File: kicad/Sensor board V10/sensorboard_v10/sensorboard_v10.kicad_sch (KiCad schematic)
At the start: 61 parts, among them J1 Conn_01x02, J10 Conn_01x04, J11 Conn_01x02, J19 Conn_01x03, J2 USB_C_Receptacle_USB2.0_14P, J20 Conn_01x02, J21 Conn_01x06, J3 Conn_01x02, J6 Conn_01x04, J7 Conn_01x04, Q1 MMBT3904, Q2 MMBT3904, SW1 SW_SPST, SW2 SW_SPST, U1 ESP32-S3-WROOM-2, U2 CH340C, U3 TJA1051T-3, U4 LM2576S-5, U5 AMS1117-3.3, U7 TXS0102DCU

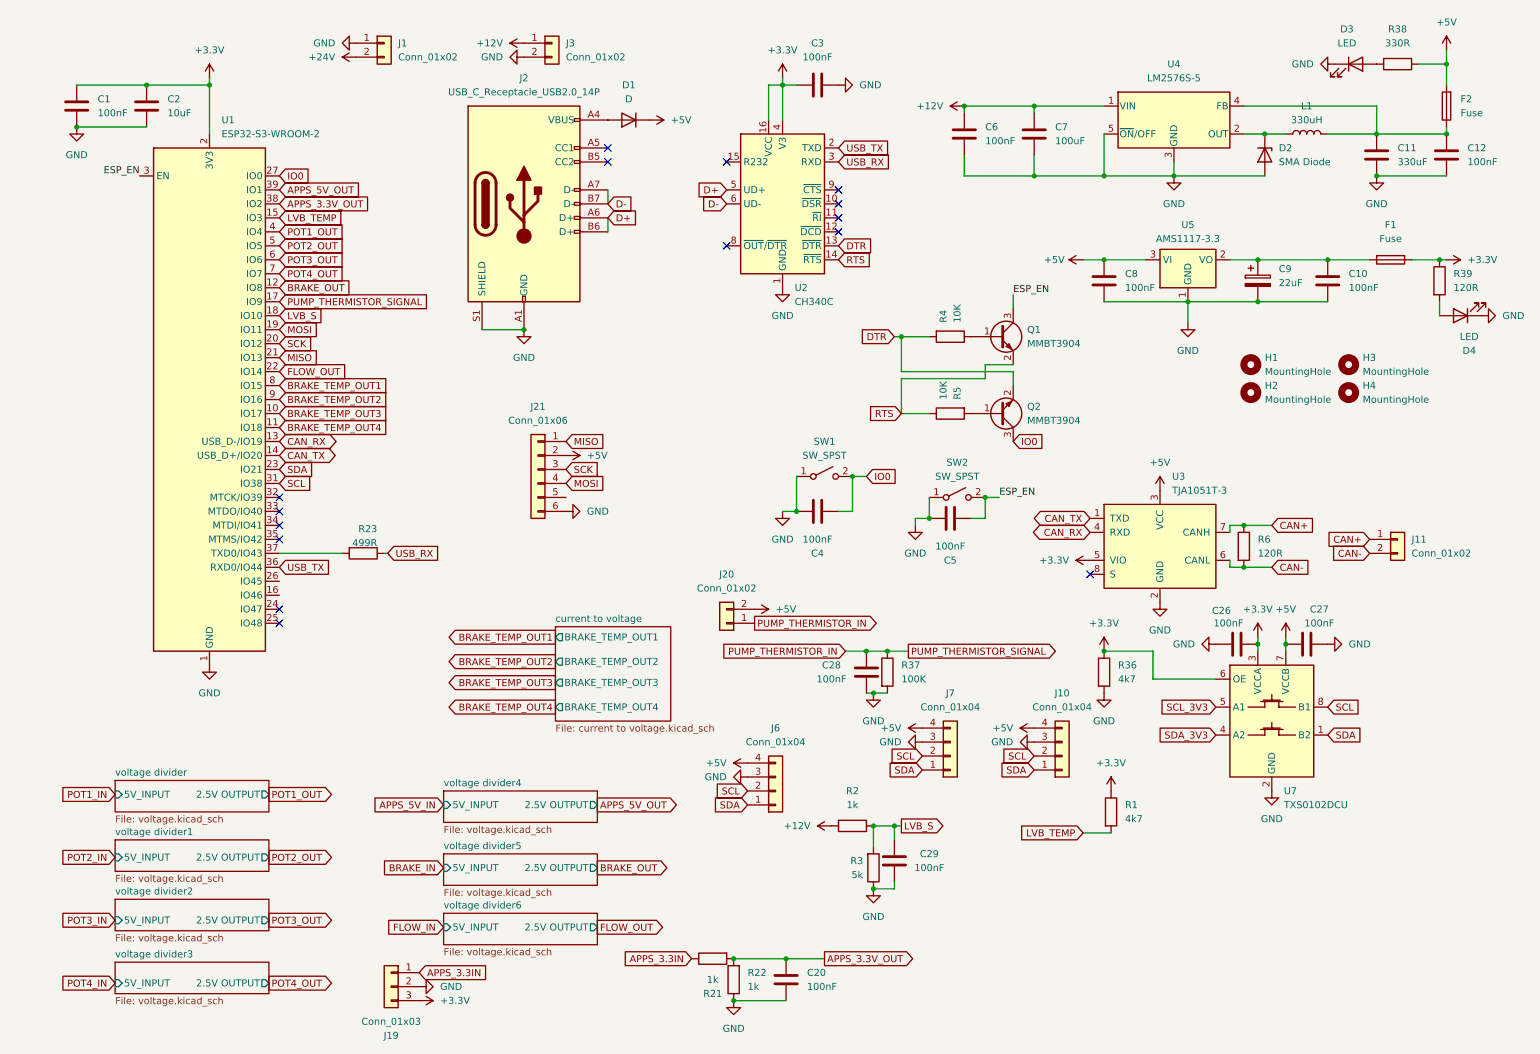
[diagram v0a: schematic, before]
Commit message: Sensor Board v10
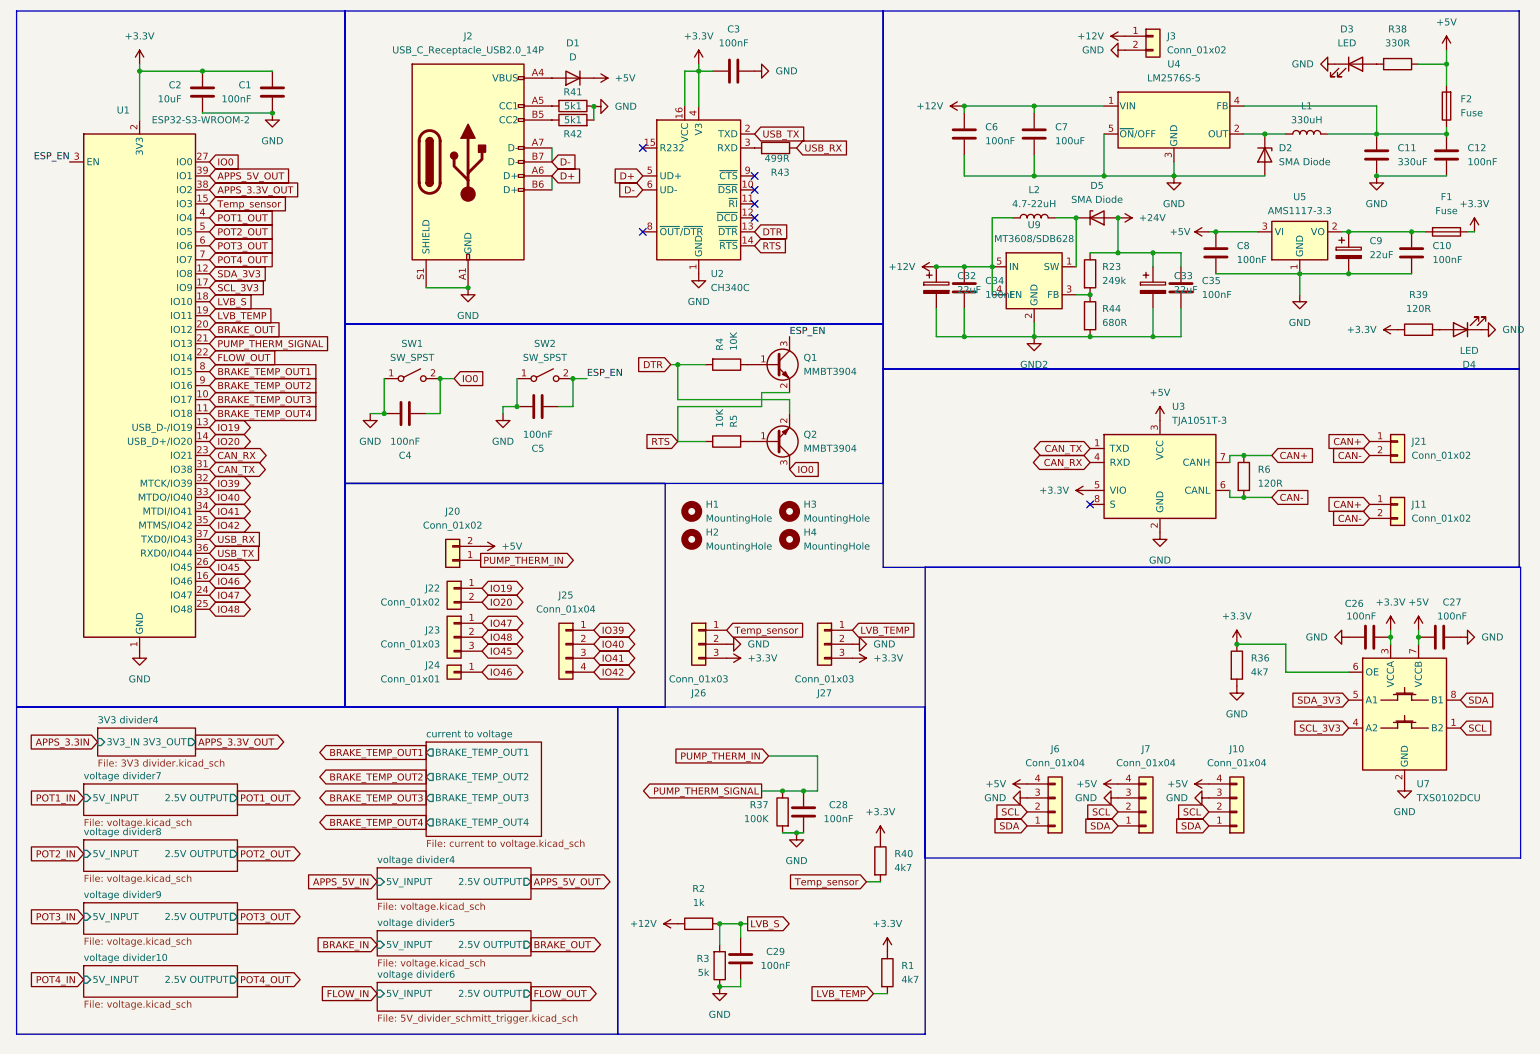
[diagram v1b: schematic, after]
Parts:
- removed C20: 100nF, RMC_Capacitor:C_0805_2012Metric_Pad1.18x1.45mm_HandSolder_L, symbol Device:C
- removed J1: Conn_01x02, Connector_JST:JST_VH_B2P-VH_1x02_P3.96mm_Vertical, symbol Connector_Generic:Conn_01x02
- removed J19: Conn_01x03, Connector_JST:JST_XH_B3B-XH-A_1x03_P2.50mm_Vertical, symbol Connector_Generic:Conn_01x03
- removed J21: Conn_01x06, Connector_PinHeader_2.54mm:PinHeader_2x03_P2.54mm_Vertical, symbol Connector_Generic:Conn_01x06
- removed R21, R22: 1k, RMC_Resistor:R_0805_2012Metric_Pad1.20x1.40mm_HandSolder_L, symbol Device:R
- added C32, C33: 22uF, RMC_Capacitor:C_0805_2012Metric_Pad1.18x1.45mm_HandSolder_L, symbol Device:C_Polarized
- added C34, C35: 100nF, RMC_Capacitor:C_0805_2012Metric_Pad1.18x1.45mm_HandSolder_L, symbol Device:C
- added D5: SMA Diode, Diode_SMD:D_SMA_Handsoldering, symbol Device:D_Zener
- added J21, J22: Conn_01x02, Connector_JST:JST_XH_B2B-XH-A_1x02_P2.50mm_Vertical, symbol Connector_Generic:Conn_01x02
- added J23, J26, J27: Conn_01x03, Connector_JST:JST_XH_B3B-XH-A_1x03_P2.50mm_Vertical, symbol Connector_Generic:Conn_01x03
- added J24: Conn_01x01, Connector_PinHeader_2.54mm:PinHeader_1x01_P2.54mm_Vertical, symbol Connector_Generic:Conn_01x01
- added J25: Conn_01x04, Connector_JST:JST_XH_B4B-XH-A_1x04_P2.50mm_Vertical, symbol Connector_Generic:Conn_01x04
- added L2: 4.7-22uH, RMC_Inductor:L_10.4x10.4_H4.8, symbol Device:L
- added R40: 4k7, RMC_Resistor:R_0805_2012Metric_Pad1.20x1.40mm_HandSolder_L, symbol Device:R
- added R41, R42: 5k1, RMC_Resistor:R_0805_2012Metric_Pad1.20x1.40mm_HandSolder_L, symbol Device:R
- added R43: 499R, RMC_Resistor:R_0805_2012Metric_Pad1.20x1.40mm_HandSolder_L, symbol Device:R
- added R44: 680R, RMC_Resistor:R_0805_2012Metric_Pad1.20x1.40mm_HandSolder_L, symbol Device:R
- added U9: MT3608/SDB628, Package_TO_SOT_SMD:SOT-23-6_Handsoldering, symbol Regulator_Switching:MT3608
- R23: value 499R -> 249k
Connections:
- net MOSI is gone; now on net LVB_TEMP: U1.19 (IO11)
- net SCK is gone; now on net BRAKE_OUT: U1.20 (IO12)
- net +12V: now also C32.1, C34.2, L2.1, U9.4 (EN), U9.5 (IN)
- net +24V: now also R23.1, C33.1, C35.2, D5.2 (A)
- net +3.3V: now also J26.3 (Pin_3), J27.3 (Pin_3), R40.1
- net BRAKE_OUT: no longer U1.12 (IO8)
- net CAN+: now also J21.1 (Pin_1)
- net CAN-: now also J21.2 (Pin_2)
- net CAN_RX: now also U1.23 (IO21); no longer U1.13 (USB_D-/IO19)
- net CAN_TX: now also U1.31 (IO38); no longer U1.14 (USB_D+/IO20)
- net GND: now also J26.2 (Pin_2), J27.2 (Pin_2), R41.1, R42.2
- net LVB_TEMP: now also J27.1 (Pin_1); no longer U1.15 (IO3)
- net SCL: now also U7.1 (B2); no longer U1.31 (IO38), U7.8 (B1)
- net SCL_3V3: now also U1.17 (IO9), U7.4 (A2); no longer U7.5 (A1)
- net SDA: now also U7.8 (B1); no longer U1.23 (IO21), U7.1 (B2)
- net SDA_3V3: now also U1.12 (IO8), U7.5 (A1); no longer U7.4 (A2)
- net USB_RX: now also U1.37 (TXD0/IO43), R43.1; no longer R23.1, U2.3 (RXD)
- net IO46: now reaches U1.16 (IO46)
- net IO46: now also J24.1 (Pin_1)
- net IO47: now reaches U1.24 (IO47)
- net IO47: now also J23.1 (Pin_1)
- net IO48: now reaches U1.25 (IO48)
- net IO48: now also J23.2 (Pin_2)
- net IO45: now reaches U1.26 (IO45)
- net IO45: now also J23.3 (Pin_3)
- net IO39: now reaches U1.32 (MTCK/IO39)
- net IO39: now also J25.1 (Pin_1)
- net IO40: now reaches U1.33 (MTDO/IO40)
- net IO40: now also J25.2 (Pin_2)
- net IO41: now reaches U1.34 (MTDI/IO41)
- net IO41: now also J25.3 (Pin_3)
- net IO42: now reaches U1.35 (MTMS/IO42)
- net IO42: now also J25.4 (Pin_4)
- net at R23.2: now also R44.1, U9.3 (FB); no longer U1.37 (TXD0/IO43)
- net at J2.A5 (CC1): now also R41.2
- net at J2.B5 (CC2): now also R42.1
- net MISO renamed PUMP_THERM_IN
- net PUMP_THERM_IN: now also C28.1, J20.1 (Pin_1), R37.1
- removed net PUMP_THERMISTOR_IN: C28.1, J20.1 (Pin_1), R37.1, U1.17 (IO9)
- new net: D5.1 (K), L2.2, U9.1 (SW)
- new net: R43.2, U2.3 (RXD)
- new net GND2: C32.2, C33.2, C34.1, C35.1, R44.2, U9.2 (GND)
- new net IO19: J22.1 (Pin_1), U1.13 (USB_D-/IO19)
- new net IO20: J22.2 (Pin_2), U1.14 (USB_D+/IO20)
- new net Temp_sensor: J26.1 (Pin_1), R40.2, U1.15 (IO3)
- no-connect marks 15 -> 7
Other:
- removed sheet voltage divider
- removed sheet voltage divider1
- removed sheet voltage divider2
- removed sheet voltage divider3
- added sheet 3V3 divider4 (3V3 divider.kicad_sch)
- added sheet voltage divider10 (voltage.kicad_sch)
- added sheet voltage divider7 (voltage.kicad_sch)
- added sheet voltage divider8 (voltage.kicad_sch)
- added sheet voltage divider9 (voltage.kicad_sch)
- sheet voltage divider6: file voltage.kicad_sch -> 5V_divider_schmitt_trigger.kicad_sch
- moved on the sheet: C1, C10, C2, C26, C27, C28, C29, C3, C4, C5, C8, C9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
